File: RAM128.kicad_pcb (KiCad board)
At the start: 4 copper layers, 71.6 x 35.7 mm, 34 parts, among them J1 AppleIIBus, U1 621024, U10 74HCT32PW, U11 74AHCT1G126GW, U2 74HCT245PW, U3 74HCT273PW, U4 74HCT273PW, U5 74HCT04PW, U6 74HCT08PW, U7 74HCT32PW, U8 74HCT08PW, U9 74HCT08PW

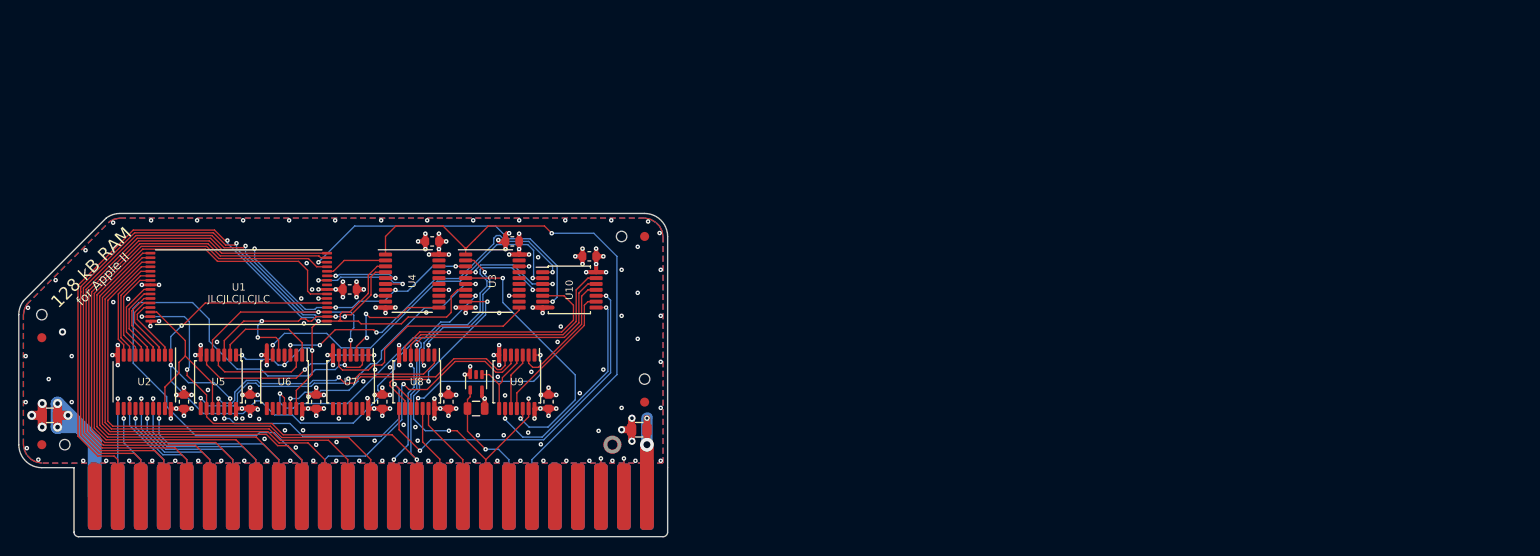
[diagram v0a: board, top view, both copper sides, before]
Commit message: done with little logic
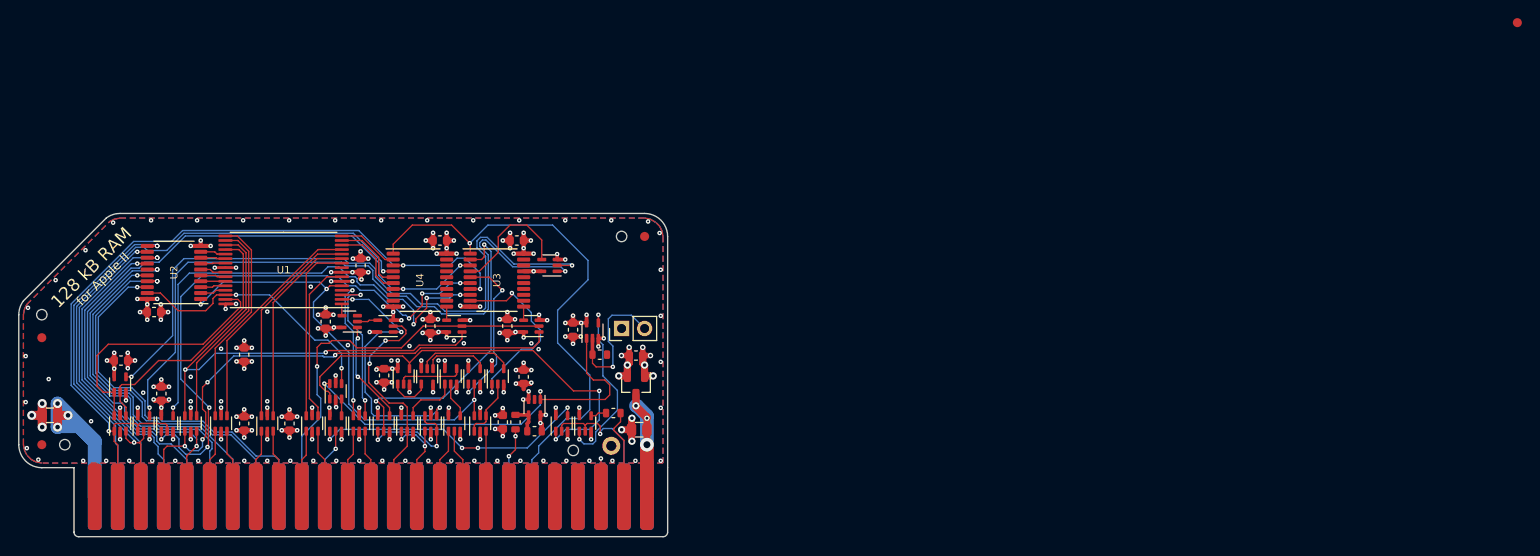
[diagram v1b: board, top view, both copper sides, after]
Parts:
- removed C1, C10, C4, C5, C6, C9: 2u2, stdpads:C_0603
- removed the C2 at (86.0, 124.8)
- removed the C8 at (115.2, 124.8)
- added C2: 2u2, stdpads:C_0603, F.Cu at (92.7, 119.6)
- added C2: 2u2, stdpads:C_0603, F.Cu at (79.1, 120.2)
- added C2: 2u2, stdpads:C_0603, F.Cu at (122.8, 107.0)
- added C2: 2u2, stdpads:C_0603, F.Cu at (105.5, 109.8)
- added C2: 2u2, stdpads:C_0603, F.Cu at (82.8, 114.9)
- added C2: 2u2, stdpads:C_0603, F.Cu at (121.2, 127.0)
- added C2: 2u2, stdpads:C_0603, F.Cu at (114.3, 107.0)
- added C2: 2u2, stdpads:C_0603, F.Cu at (92.7, 127.2)
- added C2: 2u2, stdpads:C_0603, F.Cu at (97.7, 127.2)
- added C8: 2u2, stdpads:C_0603, F.Cu at (83.5, 123.9)
- added C8: 2u2, stdpads:C_0603, F.Cu at (123.5, 122.0)
- added C8: 2u2, stdpads:C_0603, F.Cu at (101.7, 116.0)
- added C8: 2u2, stdpads:C_0603, F.Cu at (113.2, 116.5)
- added C8: 2u2, stdpads:C_0603, F.Cu at (121.8, 116.5)
- added C8: 2u2, stdpads:C_0603, F.Cu at (129.0, 116.8)
- added JP1: Disable DMA Gate, Connector_PinHeader_2.54mm:PinHeader_1x02_P2.54mm_Vertical, F.Cu at (134.4, 116.7)
- added R3: 30, stdpads:R_0603, F.Cu at (133.4, 126.0)
- added R4: 30, stdpads:R_0603, F.Cu at (122.7, 127.0)
- added R6: 3k3, stdpads:R_0603, F.Cu at (131.9, 119.6)
- added U12: 74LVC1G08GW, stdpads:SOT-353, F.Cu at (108.3, 116.5)
- added U13: 74LVC1G32GW, stdpads:SOT-353, F.Cu at (104.3, 116.0)
- added U14: 74LVC1G08GW, stdpads:SOT-353, F.Cu at (108.1, 127.2)
- added U15: 742G04GW, stdpads:SOT-363, F.Cu at (86.8, 127.2)
- added U16: 74LVC1G32GW, stdpads:SOT-353, F.Cu at (124.4, 116.5)
- added U17: 742G04GW, stdpads:SOT-363, F.Cu at (90.2, 127.2)
- added U18: 742G04GW, stdpads:SOT-363, F.Cu at (95.2, 127.2)
- added U19: 74LVC1G08GW, stdpads:SOT-353, F.Cu at (118.1, 122.0)
- added U20: 742G04GW, stdpads:SOT-363, F.Cu at (100.2, 127.2)
- added U21: 74LVC1G32GW, stdpads:SOT-353, F.Cu at (112.9, 122.0)
- added U22: 74LVC1G08GW, stdpads:SOT-353, F.Cu at (130.3, 127.2)
- added U23: 74LVC1G08GW, stdpads:SOT-353, F.Cu at (120.7, 122.0)
- added U24: 74LVC1G08GW, stdpads:SOT-353, F.Cu at (110.3, 122.0)
- added U25: 742G04GW, stdpads:SOT-363, F.Cu at (105.4, 127.2)
- added U26: 74LVC1G08GW, stdpads:SOT-353, F.Cu at (115.9, 127.2)
- added U27: 74LVC1G08GW, stdpads:SOT-353, F.Cu at (127.8, 127.2)
- added U28: 74LVC1G08GW, stdpads:SOT-353, F.Cu at (115.5, 122.0)
- added U29: 742G04GW, stdpads:SOT-363, F.Cu at (113.3, 127.2)
- added U30: 74LVC1G08GW, stdpads:SOT-353, F.Cu at (102.8, 127.2)
- added U31: 742G04GW, stdpads:SOT-363, F.Cu at (102.8, 123.7)
- added U32: 74LVC1G32GW, stdpads:SOT-353, F.Cu at (110.7, 127.2)
- added U33: 742G04GW, stdpads:SOT-363, F.Cu at (118.8, 127.2)
- added U34: 74LVC1G32GW, stdpads:SOT-353, F.Cu at (131.2, 117.0)
- added U35: XC6206PxxxMR, stdpads:SOT-23, F.Cu at (135.9, 123.0)
- R1: footprint stdpads:R_0805 -> stdpads:R_0603
- U1: footprint stdpads:TSOP-I-32_18.4x8mm_P0.5mm -> stdpads:TSOP-I-32_11.8x8mm_P0.5mm
- U10: value 74HCT32PW -> 742G04GW; footprint stdpads:TSSOP-14_4.4x5mm_P0.65mm -> stdpads:SOT-363
- U11: value 74AHCT1G126GW -> 74LVC1G125GW
- U2: value 74HCT245PW -> 74AHC245PW
- U5: value 74HCT04PW -> 74LVC1G08GW; footprint stdpads:TSSOP-14_4.4x5mm_P0.65mm -> stdpads:SOT-353
- U6, U8: value 74HCT08PW -> 74LVC1G32GW; footprint stdpads:TSSOP-14_4.4x5mm_P0.65mm -> stdpads:SOT-353
- U7: value 74HCT32PW -> 74LVC1G08GW; footprint stdpads:TSSOP-14_4.4x5mm_P0.65mm -> stdpads:SOT-353
- U9: value 74HCT08PW -> 74LVC1G08GW; footprint stdpads:TSSOP-14_4.4x5mm_P0.65mm -> stdpads:SOT-353
- moved FID4 105.1 mm to (233.2, 83.0)
- moved U10 51.7 mm to (79.0, 127.2), turned to 90 degrees
- moved U9 38.9 mm to (84.2, 127.2), turned to 270 degrees
- moved U6 31.9 mm to (126.4, 109.8), turned to 0 degrees
- moved U7 23.3 mm to (81.6, 127.2), turned to 270 degrees
- moved C3 18.6 mm to (135.9, 119.7), turned to 0 degrees
- moved U2 12.5 mm to (85.0, 110.5), turned to 90 degrees
- moved H5 11.1 mm to (129.0, 130.2)
- moved U5 10.9 mm to (79.0, 122.9), turned to 270 degrees
- moved U8 7.42 mm to (115.9, 116.5), turned to 0 degrees
- moved U11 7.01 mm to (124.8, 125.4)
- moved R1 6.92 mm to (124.8, 128.1)
- moved U1 5.30 mm to (97.0, 110.2)
- moved C7 2.91 mm to (108.2, 121.9), turned to 270 degrees
- moved U4 0.86 mm to (112.1, 111.4)
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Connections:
- C3 pad 1: +5V -> +3V3
- C7 pad 1: +5V -> +3V3
- J1 pad 24: /DMAin -> /DMAout
- R1 pad 1: +5V -> +3V3
- R1 pad 2: /~INH~ -> Net-(R1-Pad2)
- U1 pad 1: /A0 -> /RA12
- U1 pad 10: /RA16 -> /~A8
- U1 pad 11: /RA15 -> /~A7
- U1 pad 12: /RA14 -> /~A6
- U1 pad 13: /A6 -> /~A5
- U1 pad 14: /RA12 -> /RA16
- U1 pad 15: /A5 -> /RA15
- U1 pad 16: /A4 -> /RA14
- U1 pad 17: /A8 -> /~A4
- U1 pad 18: /A9 -> /~A3
- U1 pad 19: /A10 -> /~A2
- U1 pad 2: /A1 -> /RA13
- U1 pad 20: /A11 -> /~A1
- U1 pad 3: /A2 -> /~A11
- U1 pad 31: /A13 -> /~A0
- U1 pad 4: /A3 -> /~A10
- U1 pad 5: /R~W~ -> /RR~W~
- U1 pad 6: +5V -> +3V3
- U1 pad 7: /A7 -> /~A9
- U1 pad 8: +5V -> +3V3
- U10 pad 1: Net-(U10-Pad1) -> /A0
- U10 pad 2: Net-(U10-Pad2) -> GND
- U10 pad 3: /~A0XOR1~ -> /A1
- U10 pad 4: Net-(U10-Pad4) -> /~A1
- U10 pad 5: Net-(U10-Pad5) -> +3V3
- U10 pad 6: /RA12 -> /~A0
- U11 pad 1: /INHOE -> /~INHOE~
- U11 pad 4: /~INH~ -> Net-(R1-Pad2)
- U11 pad 5: +5V -> +3V3
- U2 pad 1: /R~W~ -> /RR~W~
- U2 pad 20: +5V -> +3V3
- U3 pad 17: GND -> +3V3
- U3 pad 20: +5V -> +3V3
- U4 pad 20: +5V -> +3V3
- U5 pad 1: /A0 -> /~A0
- U5 pad 2: Net-(U5-Pad2) -> /~A1
- U5 pad 3: /A1 -> GND
- U5 pad 5: /A2 -> +3V3
- U6 pad 1: Net-(U5-Pad2) -> Net-(U6-Pad1)
- U6 pad 3: Net-(U10-Pad1) -> GND
- U6 pad 4: /A0 -> /~A0XOR1~
- U6 pad 5: /A1 -> +3V3
- U7 pad 1: Net-(U5-Pad6) -> /A0
- U7 pad 2: /~DEVSEL~ -> /A1
- U7 pad 3: /A2clk -> GND
- U7 pad 4: /A2 -> Net-(U6-Pad1)
- U7 pad 5: /~DEVSEL~ -> +3V3
- U8 pad 1: Net-(U5-Pad8) -> /~A2
- U8 pad 2: /BankAB -> /~DEVSEL~
- U8 pad 3: Net-(U10-Pad4) -> GND
- U8 pad 4: /A13 -> /A2clk
- U8 pad 5: /A12 -> +3V3
- U9 pad 1: Net-(U8-Pad11) -> /ENWR1
- U9 pad 2: Net-(U10-Pad11) -> /A0
- U9 pad 3: Net-(U9-Pad10) -> GND
- U9 pad 4: /INHOE -> /ENWR1A0
- U9 pad 5: /PHI0 -> +3V3
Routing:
- net /R~W~: track 101.4 -> 7.24 mm, vias 5 -> 0
- net +3V3: track 0.00 -> 89.2 mm, vias 0 -> 87
- net Net-(U6-Pad1): track 0.00 -> 74.8 mm, vias 0 -> 2
- net /A13: track 86.2 -> 12.0 mm, vias 4 -> 2
- net /A7: track 71.1 -> 7.49 mm
- net Net-(U5-Pad4): track 11.6 -> 73.7 mm, vias 0 -> 2
- net /A6: track 67.0 -> 7.49 mm
- net /A5: track 65.1 -> 7.50 mm
- net /~A2: track 0.00 -> 56.2 mm, vias 0 -> 2
- net /A4: track 63.4 -> 7.48 mm
- net /RR~W~: track 0.00 -> 51.5 mm, vias 0 -> 3
- net /A11: track 54.5 -> 7.49 mm
- net /~INHOE~: track 0.00 -> 45.5 mm, vias 0 -> 2
- net /A10: track 52.9 -> 7.48 mm
- net /A9: track 51.3 -> 7.54 mm
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- added copper zone on In2.Cu, net +3V3
- removed copper zone on In2.Cu, net +5V
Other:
- board text removed: "JLCJLCJLCJLC"
